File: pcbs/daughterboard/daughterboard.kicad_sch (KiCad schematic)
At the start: 5 parts, among them J1 Conn_01x10_Socket, J2 Conn_01x01, J3 Conn_01x01, U1 nice_nano

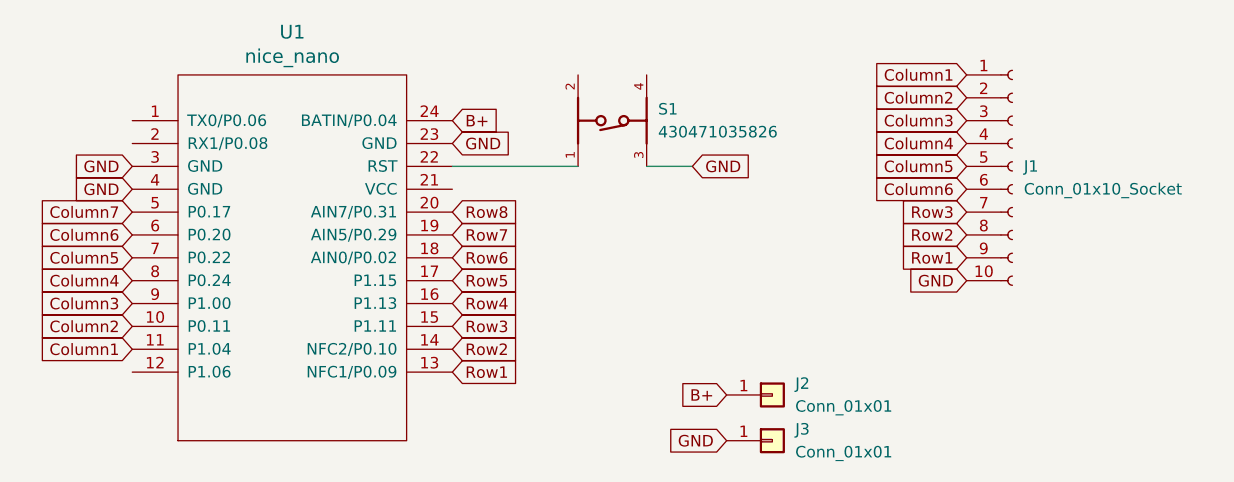
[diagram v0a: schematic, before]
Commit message: plate and pcb finished
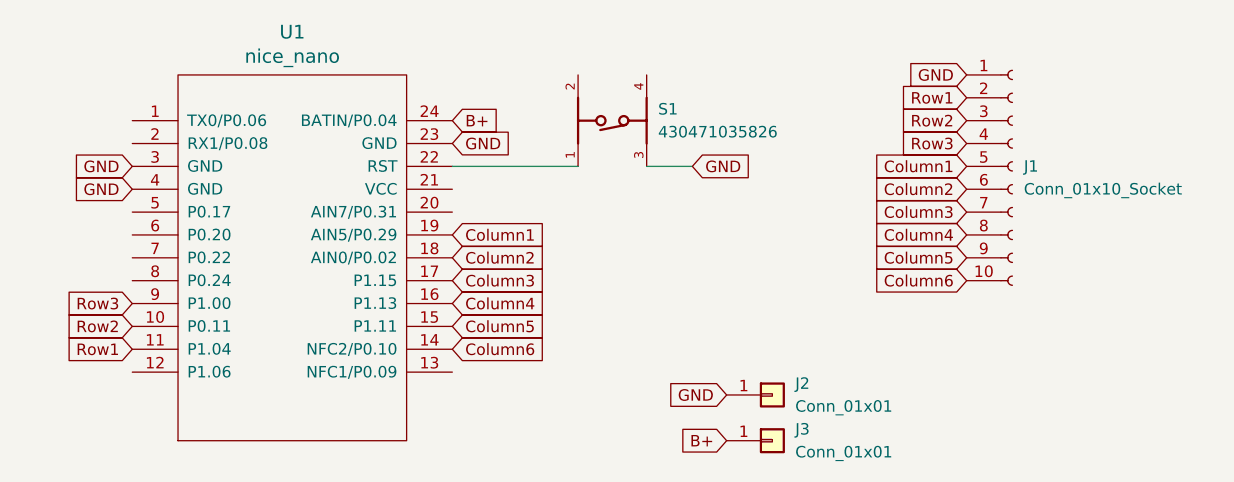
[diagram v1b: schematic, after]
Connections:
- net Row4 is gone; now on net Column4: U1.16 (P1.13)
- net Row5 is gone; now on net Column3: U1.17 (P1.15)
- net Row6 is gone; now on net Column2: U1.18 (AIN0/P0.02)
- net Row7 is gone; now on net Column1: U1.19 (AIN5/P0.29)
- net B+: now also J3.1 (Pin_1); no longer J2.1 (Pin_1)
- net Column1: now also J1.5 (Pin_5); no longer J1.1 (Pin_1), U1.11 (P1.04)
- net Column2: now also J1.6 (Pin_6); no longer J1.2 (Pin_2), U1.10 (P0.11)
- net Column3: now also J1.7 (Pin_7); no longer J1.3 (Pin_3), U1.9 (P1.00)
- net Column4: now also J1.8 (Pin_8); no longer J1.4 (Pin_4), U1.8 (P0.24)
- net Column5: now also J1.9 (Pin_9), U1.15 (P1.11); no longer J1.5 (Pin_5), U1.7 (P0.22)
- net Column6: now also J1.10 (Pin_10), U1.14 (NFC2/P0.10); no longer J1.6 (Pin_6), U1.6 (P0.20)
- net GND: now also J1.1 (Pin_1), J2.1 (Pin_1); no longer J1.10 (Pin_10), J3.1 (Pin_1)
- net Row1: now also J1.2 (Pin_2), U1.11 (P1.04); no longer J1.9 (Pin_9), U1.13 (NFC1/P0.09)
- net Row2: now also J1.3 (Pin_3), U1.10 (P0.11); no longer J1.8 (Pin_8), U1.14 (NFC2/P0.10)
- net Row3: now also J1.4 (Pin_4), U1.9 (P1.00); no longer J1.7 (Pin_7), U1.15 (P1.11)
- net Column7: no longer names the net of U1.5 (P0.17)
- net Row8: no longer names the net of U1.20 (AIN7/P0.31)
